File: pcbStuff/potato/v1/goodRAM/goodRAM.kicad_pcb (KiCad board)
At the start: 2 copper layers, 16 parts, among them U1 74HC238, U10 74LS74, U11 74LS08, U12 74LS74, U13 74LS08, U14 74LS74, U15 74LS74, U2 74HC238, U3 74LS08, U4 74LS74, U5 74LS74, U6 74LS08, U7 74LS74, U8 74LS08, U9 74LS74

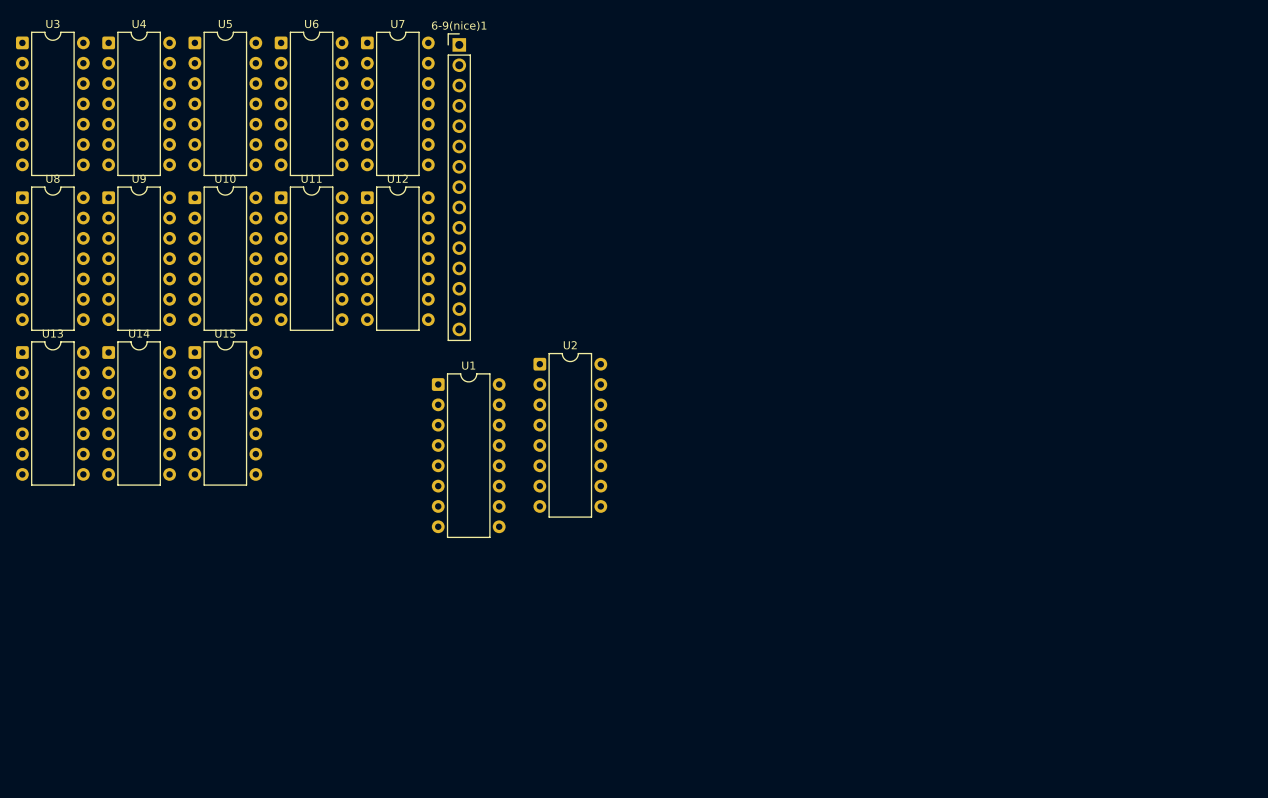
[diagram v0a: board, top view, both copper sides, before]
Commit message: im very bad
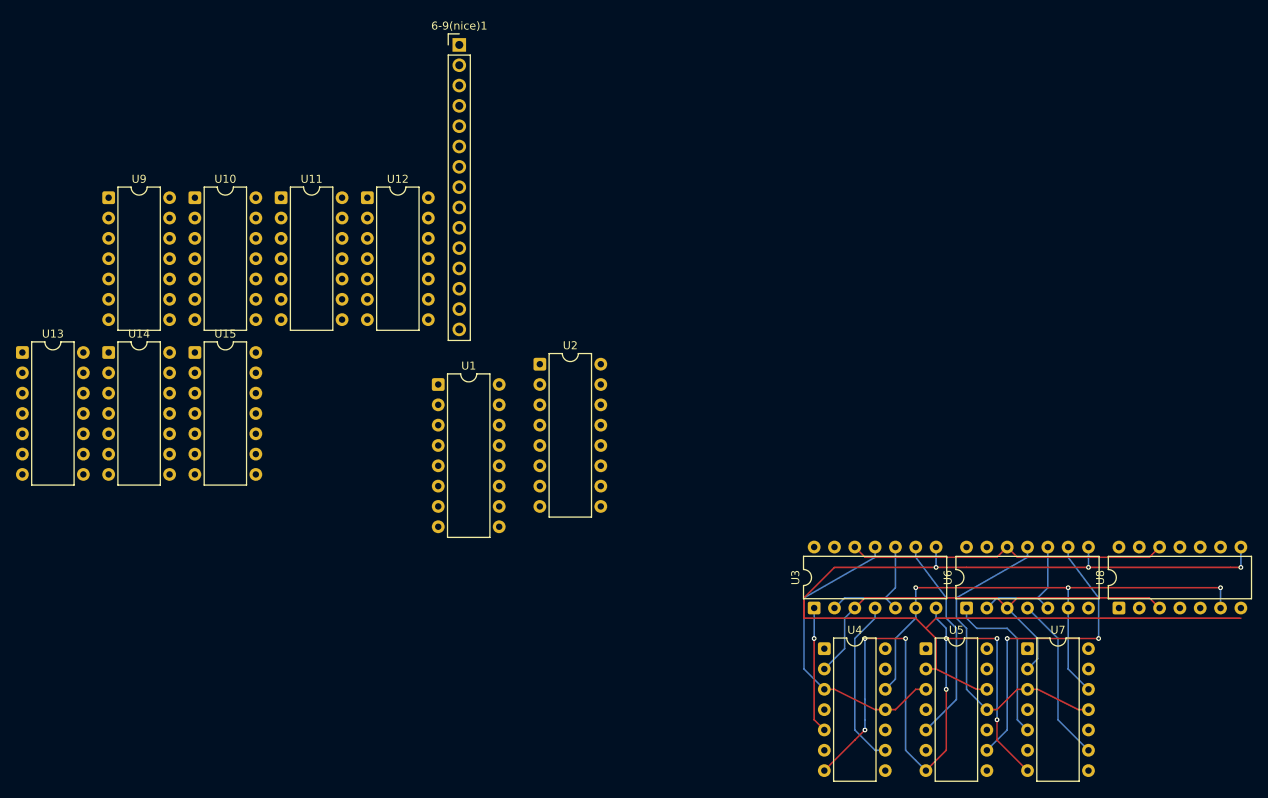
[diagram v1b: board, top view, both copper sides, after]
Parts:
- moved U8 146.4 mm to (152.4, 86.4), turned to 90 degrees
- moved U3 121.6 mm to (114.3, 86.4), turned to 90 degrees
- moved U5 118.7 mm to (128.3, 91.4)
- moved U4 117.2 mm to (115.6, 91.4)
- moved U7 112.0 mm to (141.0, 91.4)
- moved U6 111.0 mm to (133.3, 86.4), turned to 90 degrees
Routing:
- net Net-(6-9(nice)1-Bus_3): track 0.00 -> 128.9 mm, vias 0 -> 3
- net GND: track 0.00 -> 87.6 mm, vias 0 -> 7
- net Net-(6-9(nice)1-Bus_2): track 0.00 -> 68.7 mm, vias 0 -> 3
- net Net-(6-9(nice)1-Bus_1): track 0.00 -> 59.1 mm
- net Net-(6-9(nice)1-Clk): track 0.00 -> 40.2 mm
- net Net-(U5B-Q): track 0.00 -> 29.0 mm, vias 0 -> 2
- net Net-(U4B-Q): track 0.00 -> 21.2 mm
- net Net-(U7B-Q): track 0.00 -> 20.9 mm
- net Net-(U7A-Q): track 0.00 -> 20.6 mm
- net Net-(U5A-Q): track 0.00 -> 19.9 mm
- net Net-(U4A-Q): track 0.00 -> 15.8 mm, vias 0 -> 1
- net Net-(U2-Y4): track 0.00 -> 15.5 mm
- net Net-(U2-Y3): track 0.00 -> 15.5 mm
- net Net-(U5B-C): track 0.00 -> 14.3 mm
- net Net-(U4A-C): track 0.00 -> 12.5 mm
